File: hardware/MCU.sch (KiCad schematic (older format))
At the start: 21 parts, among them J301 Debug, J302 BME280, SW301 Boot option, SW302 Reset, SW303 Factory reset, U301 ESP32_WROVER, U302 TXB0102DCU

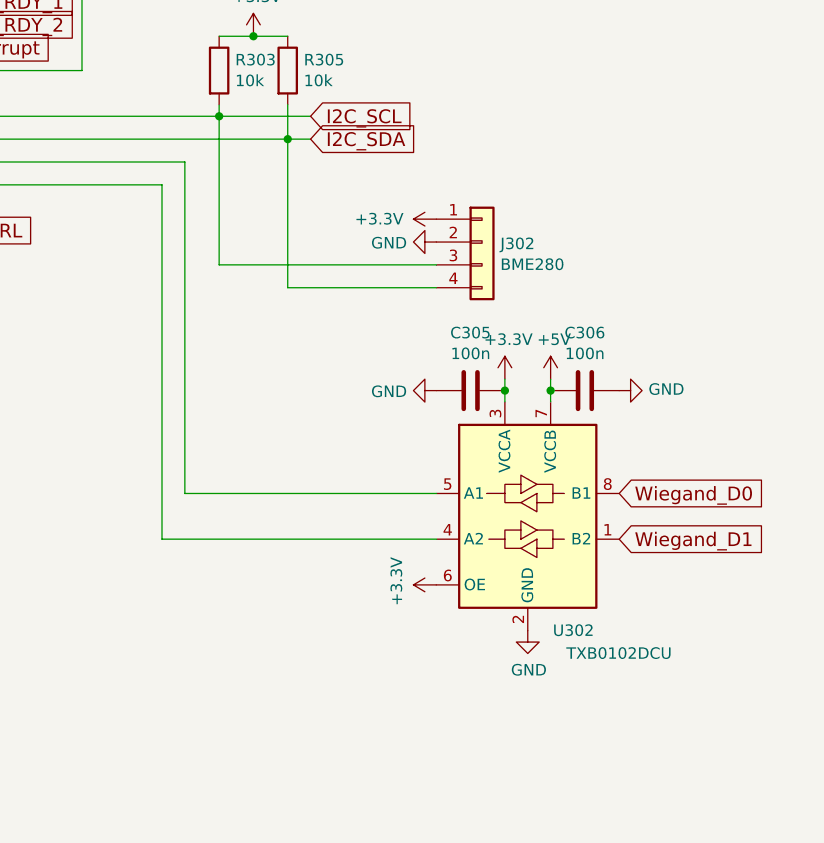
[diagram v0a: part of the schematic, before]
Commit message: Replaced TXB0102DCU with SN74LV4T125. Closes #13
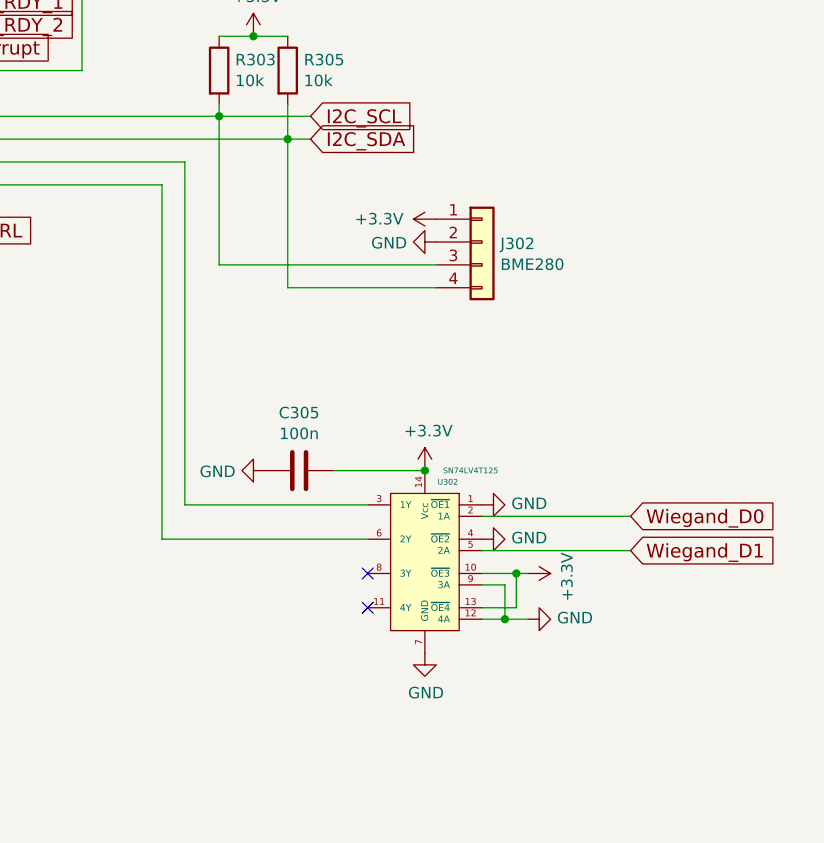
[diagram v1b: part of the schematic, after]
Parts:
- removed C306: 100n, Capacitor_SMD:C_0805_2012Metric, symbol Device:C
- removed U302: TXB0102DCU, Package_SO:VSSOP-8_2.4x2.1mm_P0.5mm, symbol Logic_LevelTranslator:TXB0102DCU
- added U302: SN74LV4T125, Package_SO:TSSOP-14_4.4x5mm_P0.65mm, symbol PerMalmberg:SN74LV4T125
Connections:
- net +3V3: now also U302.10 (~OE3), U302.13 (~OE4), U302.14 (Vcc)
- net GND: now also U302.1 (~OE1), U302.12 (4A), U302.4 (~OE2), U302.7 (GND), U302.9 (3A)
- net Wiegand_D0: now also U302.2 (1A)
- net Wiegand_D1: now also U302.5 (2A)
- net at U301.11 (GPIO26): now also U302.6 (2Y)
- net at U301.12 (GPIO27): now also U302.3 (1Y)
- no-connect marks 1 -> 3
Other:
- moved on the sheet: C305
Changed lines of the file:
@@
 	7500 2650 7650 2650
-$Comp
-L Logic_LevelTranslator:TXB0102DCU U302
-U 1 1 5B73B5D9
-P 8700 4750
-F 0 "U302" H 8900 4250 50  0000 C CNN
-F 1 "TXB0102DCU" H 9100 4150 50  0000 C CNN
-F 2 "Package_SO:VSSOP-8_2.4x2.1mm_P0.5mm" H 8700 4200 50  0001 C CNN
-F 3 "https://www.mouser.se/ProductDetail/Texas-Instruments/TXB0102DCUR?qs=sGAEpiMZZMsty6Jaj0%252bBBsMF3VbNM0929UnYQvFKVv0%3d" H 8700 4720 50  0001 C CNN
-	1    8700 4750
-	1    0    0    -1
-$EndComp
 $Comp
 L power:+3.3V #PWR0317
 U 1 1 5B73B74B
-P 8600 4150
-F 0 "#PWR0317" H 8600 4000 50  0001 C CNN
-F 1 "+3.3V" H 8615 4323 50  0000 C CNN
-F 2 "" H 8600 4150 50  0001 C CNN
-F 3 "" H 8600 4150 50  0001 C CNN
-	1    8600 4150
-	1    0    0    -1
-$EndComp
-$Comp
-L power:+5V #PWR0319
-U 1 1 5B73B784
-P 8800 4150
-F 0 "#PWR0319" H 8800 4000 50  0001 C CNN
-F 1 "+5V" H 8815 4323 50  0000 C CNN
-F 2 "" H 8800 4150 50  0001 C CNN
-F 3 "" H 8800 4150 50  0001 C CNN
-	1    8800 4150
-	1    0    0    -1
-$EndComp
-$Comp
-L Device:C C306
-U 1 1 5B73B7BC
-P 8950 4200
-F 0 "C306" V 8698 4200 50  0000 C CNN
-F 1 "100n" V 8789 4200 50  0000 C CNN
-F 2 "Capacitor_SMD:C_0805_2012Metric" H 8988 4050 50  0001 C CNN
-F 3 "https://www.mouser.se/ProductDetail/KEMET/C0805C104J5RACTU?qs=sGAEpiMZZMs0AnBnWHyRQFCCI5cSbRT%2fIwsdZoDYv9I%3d" H 8950 4200 50  0001 C CNN
-	1    8950 4200
-	0    1    1    0
+P 8250 4550
+F 0 "#PWR0317" H 8250 4400 50  0001 C CNN
+F 1 "+3.3V" H 8265 4723 50  0000 C CNN
+F 2 "" H 8250 4550 50  0001 C CNN
+F 3 "" H 8250 4550 50  0001 C CNN
+	1    8250 4550
+	1    0    0    -1
 $EndComp
 $Comp
 L Device:C C305
 U 1 1 5B73B81A
-P 8450 4200
-F 0 "C305" V 8702 4200 50  0000 C CNN
-F 1 "100n" V 8611 4200 50  0000 C CNN
-F 2 "Capacitor_SMD:C_0805_2012Metric" H 8488 4050 50  0001 C CNN
-F 3 "https://www.mouser.se/ProductDetail/KEMET/C0805C104J5RACTU?qs=sGAEpiMZZMs0AnBnWHyRQFCCI5cSbRT%2fIwsdZoDYv9I%3d" H 8450 4200 50  0001 C CNN
-	1    8450 4200
-	0    -1   -1   0
-$EndComp
-Wire Wire Line
-	8600 4250 8600 4200
-Connection ~ 8600 4200
-Wire Wire Line
-	8600 4200 8600 4150
-Wire Wire Line
-	8800 4150 8800 4200
-Connection ~ 8800 4200
-Wire Wire Line
-	8800 4200 8800 4250
+P 7700 4550
+F 0 "C305" V 7952 4550 50  0000 C CNN
+F 1 "100n" V 7861 4550 50  0000 C CNN
+F 2 "Capacitor_SMD:C_0805_2012Metric" H 7738 4400 50  0001 C CNN
+F 3 "https://www.mouser.se/ProductDetail/KEMET/C0805C104J5RACTU?qs=sGAEpiMZZMs0AnBnWHyRQFCCI5cSbRT%2fIwsdZoDYv9I%3d" H 7700 4550 50  0001 C CNN
+	1    7700 4550
+	0    -1   -1   0
+$EndComp
 $Comp
 L power:GND #PWR0314
 U 1 1 5B73C2C7
-P 8300 4200
-F 0 "#PWR0314" H 8300 3950 50  0001 C CNN
-F 1 "GND" V 8305 4072 50  0000 R CNN
-F 2 "" H 8300 4200 50  0001 C CNN
-F 3 "" H 8300 4200 50  0001 C CNN
-	1    8300 4200
-	0    1    1    0
-$EndComp
-$Comp
-L power:GND #PWR0320
-U 1 1 5B73C2E7
-P 9100 4200
-F 0 "#PWR0320" H 9100 3950 50  0001 C CNN
-F 1 "GND" V 9105 4072 50  0000 R CNN
-F 2 "" H 9100 4200 50  0001 C CNN
-F 3 "" H 9100 4200 50  0001 C CNN
-	1    9100 4200
-	0    -1   -1   0
-$EndComp
-Text GLabel 9100 4650 2    60   Input ~ 0
+P 7550 4550
+F 0 "#PWR0314" H 7550 4300 50  0001 C CNN
+F 1 "GND" V 7555 4422 50  0000 R CNN
+F 2 "" H 7550 4550 50  0001 C CNN
+F 3 "" H 7550 4550 50  0001 C CNN
+	1    7550 4550
+	0    1    1    0
+$EndComp
+Text GLabel 9150 4750 2    60   Input ~ 0
 Wiegand_D0
-Text GLabel 9100 4850 2    60   Input ~ 0
+Text GLabel 9150 4900 2    60   Input ~ 0
 Wiegand_D1
 $Comp
 L power:GND #PWR0318
 U 1 1 5B73CB5F
-P 8700 5250
-F 0 "#PWR0318" H 8700 5000 50  0001 C CNN
-F 1 "GND" H 8705 5077 50  0000 C CNN
-F 2 "" H 8700 5250 50  0001 C CNN
-F 3 "" H 8700 5250 50  0001 C CNN
-	1    8700 5250
+P 8250 5350
+F 0 "#PWR0318" H 8250 5100 50  0001 C CNN
+F 1 "GND" H 8255 5177 50  0000 C CNN
+F 2 "" H 8250 5350 50  0001 C CNN
+F 3 "" H 8250 5350 50  0001 C CNN
+	1    8250 5350
 	1    0    0    -1
 $EndComp
@@
 DIA_Interrupt
 Wire Wire Line
-	8300 4650 7200 4650
-Wire Wire Line
-	7200 4650 7200 3200
-Wire Wire Line
 	7200 3200 5450 3200
 Wire Wire Line
@@
 Wire Wire Line
 	7100 3300 7100 4850
-Wire Wire Line
-	7100 4850 8300 4850
 Wire Wire Line
 	5450 2800 6750 2800
@@
 	1500 3400 1300 3400
 $Comp
-L power:+3.3V #PWR0101
-U 1 1 5BF7E862
-P 8300 5050
-F 0 "#PWR0101" H 8300 4900 50  0001 C CNN
-F 1 "+3.3V" H 8315 5223 50  0000 C CNN
-F 2 "" H 8300 5050 50  0001 C CNN
-F 3 "" H 8300 5050 50  0001 C CNN
-	1    8300 5050
-	0    -1   -1   0
-$EndComp
+L PerMalmberg:SN74LV4T125 U302
+U 1 1 5C354023
+P 8250 4950
+F 0 "U302" H 8150 5300 25  0000 C CNN
+F 1 "SN74LV4T125" H 8050 5350 25  0000 C CNN
+F 2 "Package_SO:TSSOP-14_4.4x5mm_P0.65mm" H 8250 5100 25  0001 C CNN
+F 3 "https://www.mouser.se/ProductDetail/Texas-Instruments/SN74LV4T125PWR?qs=%2fha2pyFadugYV45CGqyCh31QZ8Sm4vmCO1dOWib7XM4PoqVfwyI%2fZw%3d%3d" H 8250 5100 25  0001 C CNN
+	1    8250 4950
+	-1   0    0    -1
+$EndComp
+Wire Wire Line
+	7200 3200 7200 4700
+Wire Wire Line
+	7200 4700 8000 4700
+Wire Wire Line
+	7100 4850 8000 4850
+Wire Wire Line
+	7850 4550 8250 4550
+Connection ~ 8250 4550
+$Comp
+L power:GND #PWR0321
+U 1 1 5C370BCE
+P 8700 5200
+F 0 "#PWR0321" H 8700 4950 50  0001 C CNN
+F 1 "GND" V 8705 5072 50  0000 R CNN
+F 2 "" H 8700 5200 50  0001 C CNN
+F 3 "" H 8700 5200 50  0001 C CNN
+	1    8700 5200
+	0    -1   -1   0
+$EndComp
+$Comp
+L power:+3.3V #PWR0320
+U 1 1 5C370C51
+P 8700 5000
+F 0 "#PWR0320" H 8700 4850 50  0001 C CNN
+F 1 "+3.3V" H 8715 5173 50  0000 C CNN
+F 2 "" H 8700 5000 50  0001 C CNN
+F 3 "" H 8700 5000 50  0001 C CNN
+	1    8700 5000
+	0    1    1    0
+$EndComp
+Wire Wire Line
+	8700 5200 8600 5200
+Wire Wire Line
+	8500 5050 8600 5050
+Wire Wire Line
+	8600 5050 8600 5200
+Connection ~ 8600 5200
+Wire Wire Line
+	8600 5200 8500 5200
+Wire Wire Line
+	8500 5000 8650 5000
+Wire Wire Line
+	8650 5000 8650 5150
+Wire Wire Line
+	8650 5150 8500 5150
+Connection ~ 8650 5000
+Wire Wire Line
+	8650 5000 8700 5000
+Wire Wire Line
+	9150 4750 8500 4750
+Wire Wire Line
+	9150 4900 8500 4900
+$Comp
+L power:GND #PWR0319
+U 1 1 5C37C6A4
+P 8500 4850
+F 0 "#PWR0319" H 8500 4600 50  0001 C CNN
+F 1 "GND" V 8505 4722 50  0000 R CNN
+F 2 "" H 8500 4850 50  0001 C CNN
+F 3 "" H 8500 4850 50  0001 C CNN
+	1    8500 4850
+	0    -1   -1   0
+$EndComp
+$Comp
+L power:GND #PWR0310
+U 1 1 5C37C6DB
+P 8500 4700
+F 0 "#PWR0310" H 8500 4450 50  0001 C CNN
+F 1 "GND" V 8505 4572 50  0000 R CNN
+F 2 "" H 8500 4700 50  0001 C CNN
+F 3 "" H 8500 4700 50  0001 C CNN
+	1    8500 4700
+	0    -1   -1   0
+$EndComp
+NoConn ~ 8000 5000
+NoConn ~ 8000 5150
 $EndSCHEMATC
